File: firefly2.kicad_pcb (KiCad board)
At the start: 2 copper layers, 41 x 41 mm, 16 parts, among them J1 10118194-0001LF, P2 CONN_01X03, P3 CONN_01X04, P4 CONN_01X05, P5 CONN_01X01, U1 SAM_D11C, U2 RFM69CW, U3 MIC5504

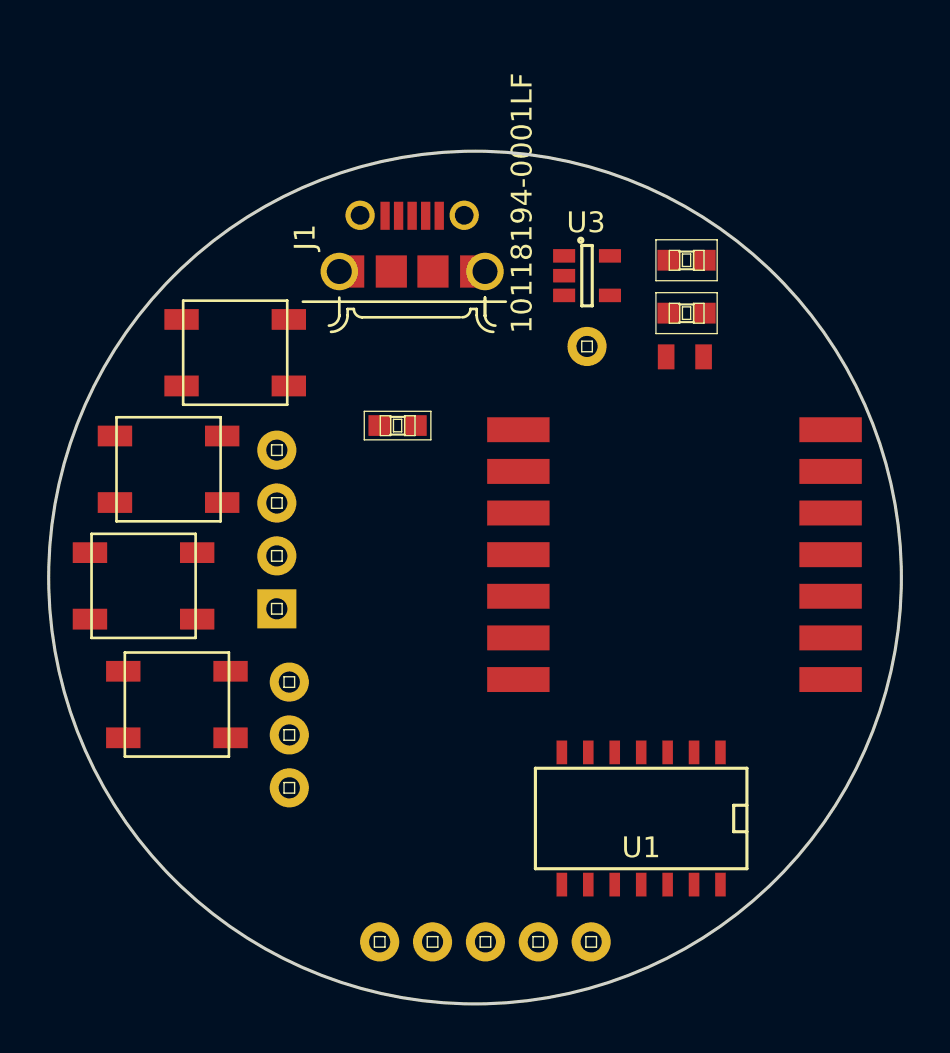
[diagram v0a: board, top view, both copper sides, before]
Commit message: Finish routing the board
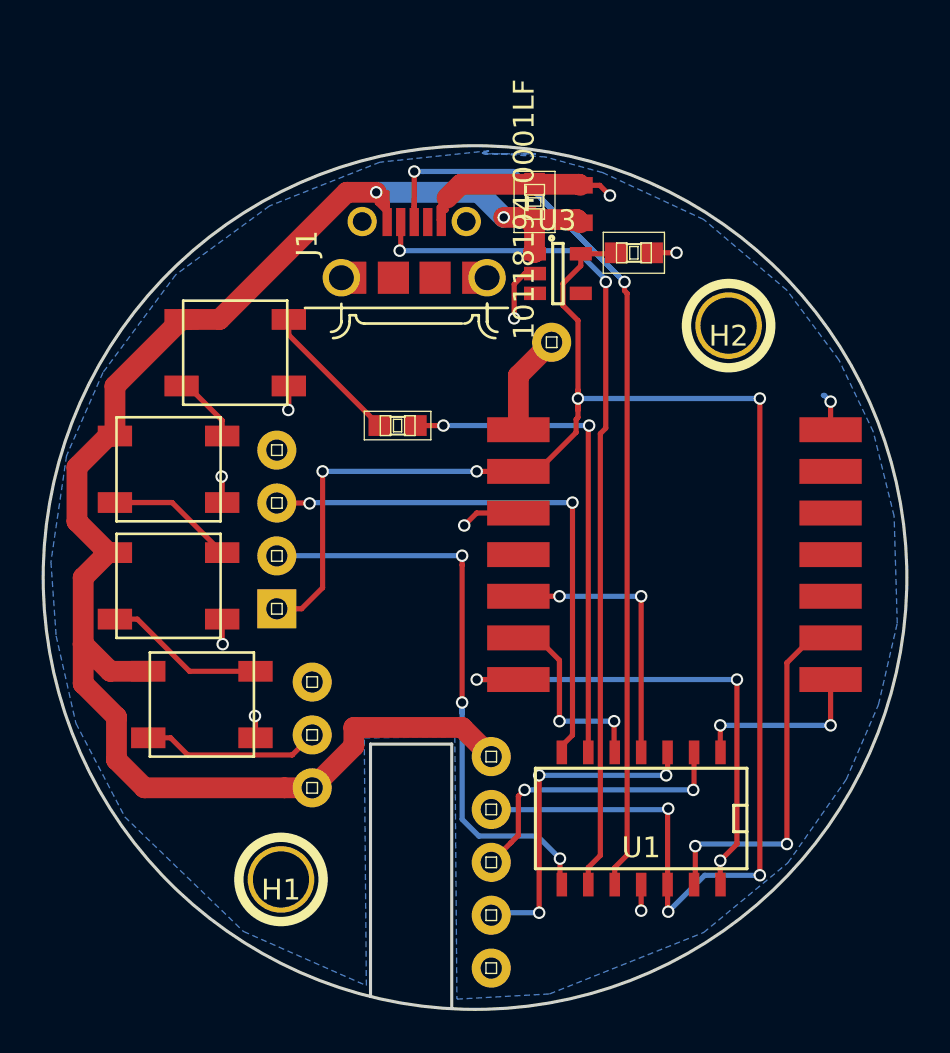
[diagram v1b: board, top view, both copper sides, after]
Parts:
- added H1: hole, homebrew:hole-m2.5, F.Cu at (150.7, 78.0)
- added H2: hole, homebrew:hole-m2.5, F.Cu at (172.2, 51.4)
- moved P4 10.1 mm to (160.8, 72.1), turned to 270 degrees
- moved C2 9.05 mm to (162.9, 45.5), turned to 270 degrees
- moved C1 8.89 mm to (165.1, 45.6), turned to 270 degrees
- moved C3 2.56 mm to (167.6, 47.9)
- moved P5 1.71 mm to (163.7, 52.2)
- moved U3 1.40 mm to (164.0, 48.9)
- moved D3 1.20 mm to (145.3, 63.9)
- moved D4 1.20 mm to (146.9, 69.6)
- moved P2 1.10 mm to (152.2, 73.6)
- moved J1 0.32 mm to (157.1, 49.1)
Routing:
- net +3V3: track 0.00 -> 84.6 mm, vias 0 -> 7
- net +5V: track 0.00 -> 77.9 mm, vias 0 -> 2
- net USB_D+: track 0.00 -> 50.0 mm, vias 0 -> 2
- net USB_D-: track 0.00 -> 41.3 mm, vias 0 -> 2
- net ARM_SWDIO: track 0.00 -> 28.6 mm, vias 0 -> 3
- net GND: track 0.00 -> 26.5 mm, vias 0 -> 10
- net ARM_SWCLK: track 0.00 -> 26.4 mm, vias 0 -> 2
- net RADIO_NSS: track 0.00 -> 24.7 mm, vias 0 -> 3
- net LED_INTERNAL: track 0.00 -> 24.1 mm, vias 0 -> 2
- net RADIO_DIO0: track 0.00 -> 17.6 mm, vias 0 -> 2
- net AUX2: track 0.00 -> 16.2 mm, vias 0 -> 3
- net AUX1: track 0.00 -> 14.1 mm, vias 0 -> 2
- net RADIO_MOSI: track 0.00 -> 13.4 mm, vias 0 -> 2
- net RADIO_SCK: track 0.00 -> 9.48 mm, vias 0 -> 2
- net RADIO_MISO: track 0.00 -> 8.80 mm, vias 0 -> 2
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- added copper zone on B.Cu, net GND
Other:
- board size 41 x 41 mm -> 41.5 x 41.5 mm
- rule trace_min: 0.2 -> 0.16
